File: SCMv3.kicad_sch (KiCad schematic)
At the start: 117 parts, among them IC1 40106, IC2 40106, IC3 TL082, J1 ISP, J1-OUT8 JACK-MONO-SWB, J2 Conn_01x02, J2-OUT7 JACK-MONO-SWB, J3 POWER, J3-OUT6 JACK-MONO-SWB, J4-OUT5 JACK-MONO-SWB, J5-OUT4 JACK-MONO-SWB, J6-OUT3 JACK-MONO-SWB, J7-OUT2 JACK-MONO-SWB, J8-OUT1 JACK-MONO-SWB, J9-CLK_IN1 JCLK_IN, Q1 Si2318, Q2 Si2318, Q3 Si2318, Q4 Si2318, U1 ATmega328-A, Y1 16MHz_18pF_FA238

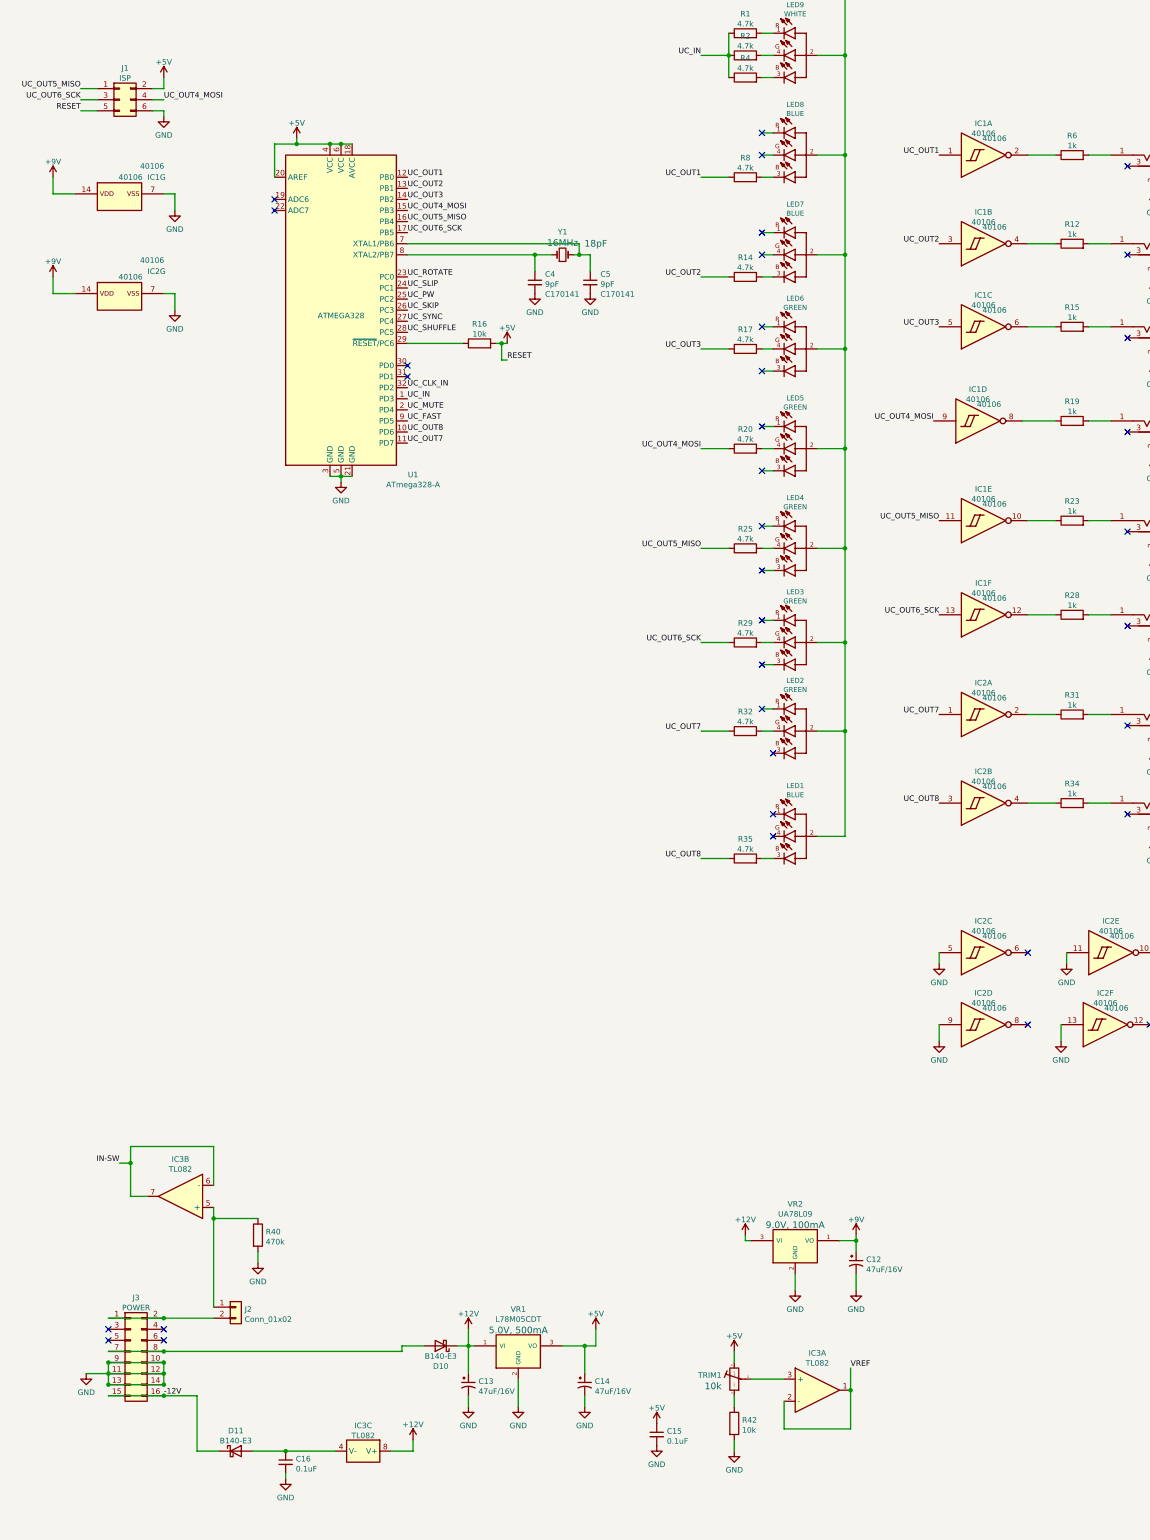
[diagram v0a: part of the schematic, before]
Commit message: PCB +SCHEM 7/02
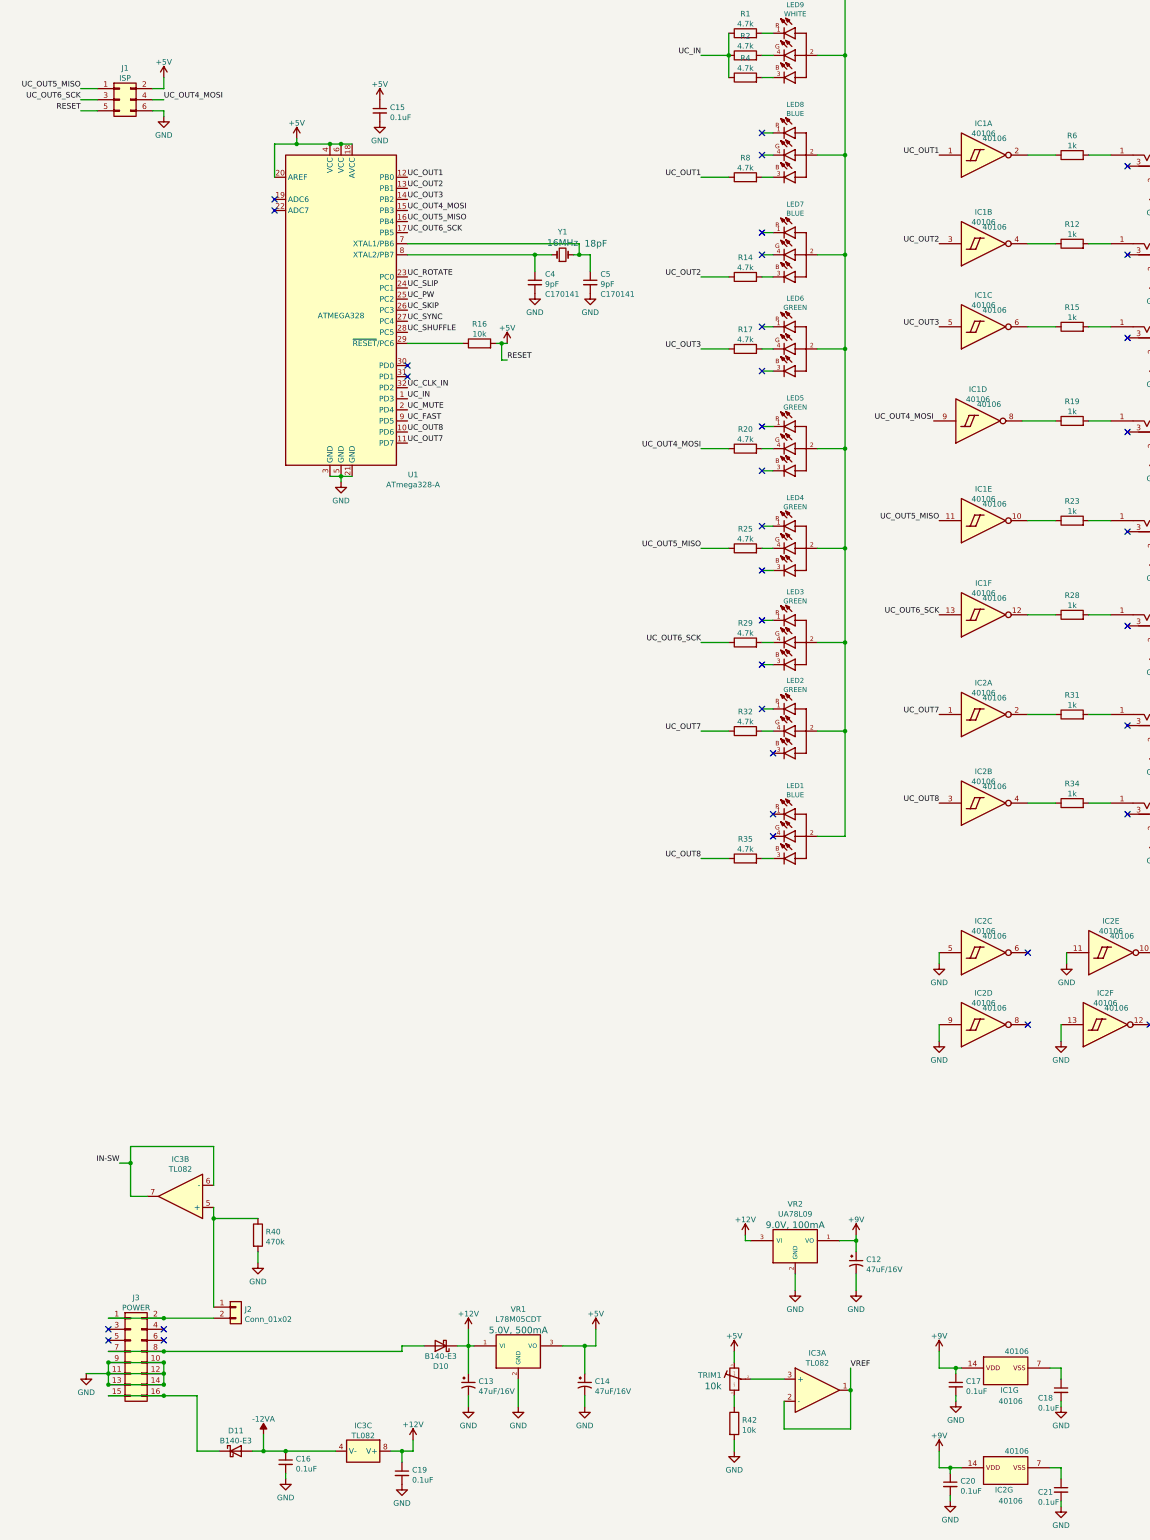
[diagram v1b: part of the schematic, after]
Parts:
- added C17, C18, C19, C20, C21: 0.1uF_0603_16V, 4ms_Capacitor:C_0603, symbol 4ms_Capacitor:0.1uF_0603_16V
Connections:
- net +12V: now also C19.1
- net +9V: now also C17.1, C20.1
- net GND: now also C17.2, C18.2, C19.2, C20.2, C21.2; no longer IC1.7 (VSS), IC2.7 (VSS)
- net -12VA: now reaches C16.1, D11.2 (A), IC3.4 (V-)
- net -12V: no longer names the net of D11.1 (K), J3.15 (-12V), J3.16 (P16)
- new net: C21.1, IC2.7 (VSS)
- new net: C18.1, IC1.7 (VSS)
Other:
- moved on the sheet: C15, IC1G, IC2G
